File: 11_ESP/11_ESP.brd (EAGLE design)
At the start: 67.4 x 44.8 mm, 8 parts, among them T1 BC847, T2 BC847, X1 ALLSERIALSLAVE

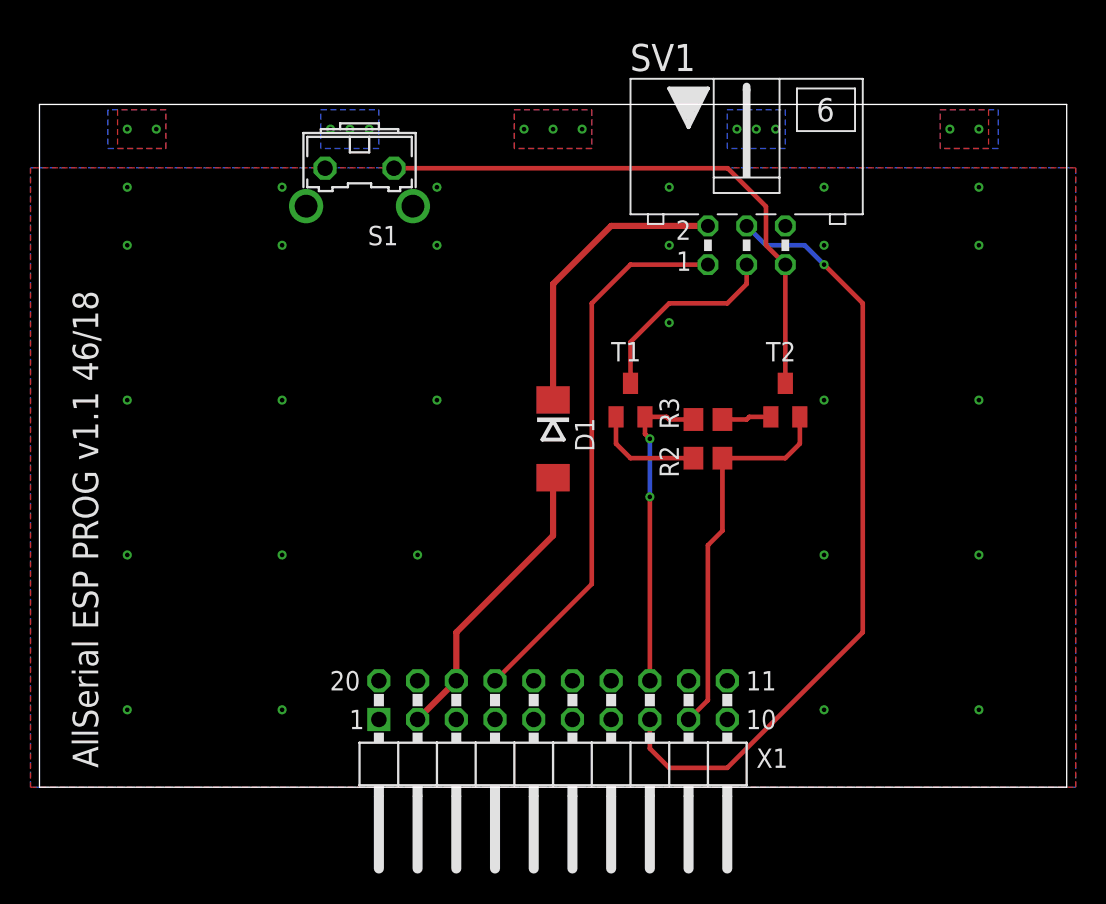
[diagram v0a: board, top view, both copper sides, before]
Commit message: Use lib elements
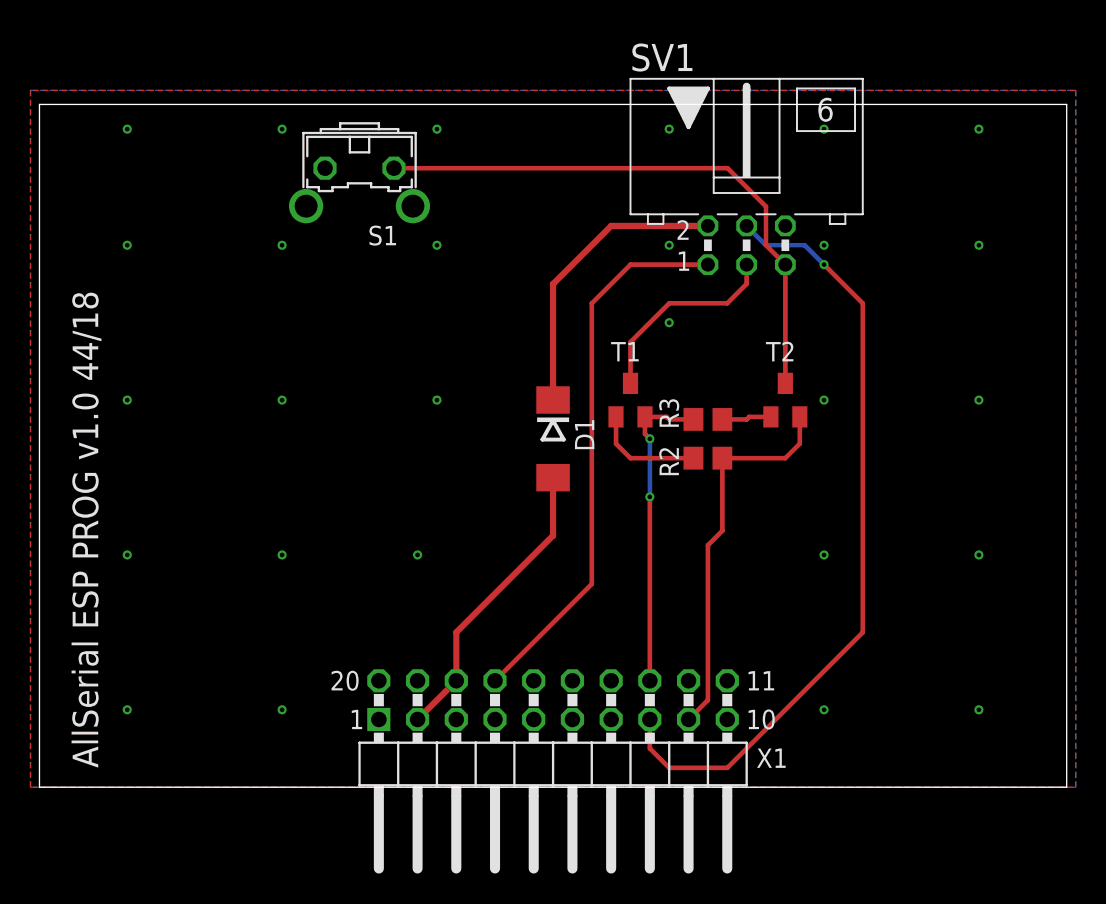
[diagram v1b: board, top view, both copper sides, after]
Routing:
- removed copper zone on layer 16, net N$10
- removed copper zone on layer 16, net N$11
- removed copper zone on layer 1, net N$13
- removed copper zone on layer 16, net N$13
- removed copper zone on layer 1, net N$14
- removed copper zone on layer 16, net N$14
- removed copper zone on layer 1, net N$15
- removed copper zone on layer 16, net N$15
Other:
- board text added: "AllSerial ESP PROG v1.0 44/18"
- board text removed: "AllSerial ESP PROG v1.1 46/18"
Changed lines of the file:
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@@
 <?xml version="1.0" encoding="utf-8"?>
 <!DOCTYPE eagle SYSTEM "eagle.dtd">
-<eagle version="7.7.0">
+<eagle version="7.6.0">
 <drawing>
 <settings>
@@
 <grid distance="1.27" unitdist="mm" unit="mm" style="lines" multiple="1" display="yes" altdistance="0.025" altunitdist="inch" altunit="inch"/>
 <layers>
-<layer number="1" name="Top" color="4" fill="1" visible="yes" active="yes"/>
+<layer number="1" name="Top" color="4" fill="1" visible="no" active="yes"/>
 <layer number="2" name="Route2" color="1" fill="3" visible="no" active="no"/>
 <layer number="3" name="Route3" color="4" fill="3" visible="no" active="no"/>
@@
 <layer number="14" name="Route14" color="1" fill="6" visible="no" active="no"/>
 <layer number="15" name="Route15" color="4" fill="6" visible="no" active="no"/>
-<layer number="16" name="Bottom" color="1" fill="1" visible="yes" active="yes"/>
+<layer number="16" name="Bottom" color="1" fill="1" visible="no" active="yes"/>
 <layer number="17" name="Pads" color="2" fill="1" visible="yes" active="yes"/>
-<layer number="18" name="Vias" color="2" fill="1" visible="yes" active="yes"/>
+<layer number="18" name="Vias" color="2" fill="1" visible="no" active="yes"/>
 <layer number="19" name="Unrouted" color="6" fill="1" visible="yes" active="yes"/>
 <layer number="20" name="Dimension" color="15" fill="1" visible="yes" active="yes"/>
@@
 <layer number="24" name="bOrigins" color="15" fill="1" visible="no" active="yes"/>
 <layer number="25" name="tNames" color="7" fill="1" visible="yes" active="yes"/>
-<layer number="26" name="bNames" color="7" fill="1" visible="yes" active="yes"/>
+<layer number="26" name="bNames" color="7" fill="1" visible="no" active="yes"/>
 <layer number="27" name="tValues" color="7" fill="1" visible="yes" active="yes"/>
 <layer number="28" name="bValues" color="7" fill="1" visible="no" active="yes"/>
-<layer number="29" name="tStop" color="7" fill="3" visible="yes" active="yes"/>
-<layer number="30" name="bStop" color="7" fill="6" visible="yes" active="yes"/>
+<layer number="29" name="tStop" color="7" fill="3" visible="no" active="yes"/>
+<layer number="30" name="bStop" color="7" fill="6" visible="no" active="yes"/>
 <layer number="31" name="tCream" color="7" fill="4" visible="no" active="yes"/>
 <layer number="32" name="bCream" color="7" fill="5" visible="no" active="yes"/>
@@
 <board>
 <plain>
-<text x="-29.845" y="1.27" size="1.6764" layer="21" rot="R90">AllSerial ESP PROG v1.1 46/18</text>
-<polygon width="0.254" layer="29">
-<vertex x="-25.4" y="44.45"/>
-<vertex x="-28.575" y="44.45"/>
-<vertex x="-28.575" y="41.91"/>
-<vertex x="-25.4" y="41.91"/>
-</polygon>
-<polygon width="0.254" layer="29">
-<vertex x="-2.54" y="44.45"/>
-<vertex x="2.54" y="44.45"/>
-<vertex x="2.54" y="41.91"/>
-<vertex x="-2.54" y="41.91"/>
-</polygon>
-<polygon width="0.254" layer="29">
-<vertex x="25.4" y="44.45"/>
-<vertex x="28.575" y="44.45"/>
-<vertex x="28.575" y="41.91"/>
-<vertex x="25.4" y="41.91"/>
-</polygon>
-<polygon width="0.254" layer="30">
-<vertex x="-29.21" y="44.45"/>
-<vertex x="-25.4" y="44.45"/>
-<vertex x="-25.4" y="41.91"/>
-<vertex x="-29.21" y="41.91"/>
-</polygon>
-<polygon width="0.254" layer="30">
-<vertex x="-15.24" y="44.45"/>
-<vertex x="-11.43" y="44.45"/>
-<vertex x="-11.43" y="41.91"/>
-<vertex x="-15.24" y="41.91"/>
-</polygon>
-<polygon width="0.254" layer="30">
-<vertex x="-2.54" y="44.45"/>
-<vertex x="2.54" y="44.45"/>
-<vertex x="2.54" y="41.91"/>
-<vertex x="-2.54" y="41.91"/>
-</polygon>
-<polygon width="0.254" layer="30">
-<vertex x="11.43" y="44.45"/>
-<vertex x="15.24" y="44.45"/>
-<vertex x="15.24" y="41.91"/>
-<vertex x="11.43" y="41.91"/>
-</polygon>
-<polygon width="0.254" layer="30">
-<vertex x="25.4" y="44.45"/>
-<vertex x="29.21" y="44.45"/>
-<vertex x="29.21" y="41.91"/>
-<vertex x="25.4" y="41.91"/>
-</polygon>
+<text x="-29.845" y="1.27" size="1.6764" layer="21" rot="R90">AllSerial ESP PROG v1.0 44/18</text>
+<rectangle x1="-8.89" y1="43.815" x2="-3.81" y2="45.72" layer="29"/>
+<rectangle x1="-25.4" y1="43.815" x2="-20.32" y2="45.72" layer="29"/>
+<rectangle x1="-1.27" y1="43.815" x2="3.81" y2="45.72" layer="29"/>
+<rectangle x1="21.59" y1="43.815" x2="26.67" y2="45.72" layer="29"/>
+<rectangle x1="-2.54" y1="43.815" x2="2.54" y2="45.72" layer="30"/>
+<rectangle x1="-12.7" y1="43.815" x2="-7.62" y2="45.72" layer="30"/>
+<rectangle x1="-22.86" y1="43.815" x2="-17.78" y2="45.72" layer="30"/>
+<rectangle x1="7.62" y1="43.815" x2="12.7" y2="45.72" layer="30"/>
+<rectangle x1="17.78" y1="43.815" x2="22.86" y2="45.72" layer="30"/>
 </plain>
 <attributes>
@@
 <signal name="GND">
 <polygon width="0.254" layer="16">
-<vertex x="-34.29" y="40.64"/>
-<vertex x="34.29" y="40.64"/>
+<vertex x="-34.29" y="45.72"/>
+<vertex x="34.29" y="45.72"/>
 <vertex x="34.29" y="0"/>
 <vertex x="-34.29" y="0"/>
@@
 <vertex x="-34.29" y="0"/>
 <vertex x="34.29" y="0"/>
-<vertex x="34.29" y="40.64"/>
-<vertex x="-34.29" y="40.64"/>
+<vertex x="34.29" y="45.72"/>
+<vertex x="-34.29" y="45.72"/>
 </polygon>
 <contactref element="X1" pad="1"/>
-<via x="-7.62" y="39.37" extent="1-16" drill="0.3"/>
-<via x="-17.78" y="39.37" extent="1-16" drill="0.3"/>
-<via x="-27.94" y="39.37" extent="1-16" drill="0.3"/>
+<via x="-7.62" y="43.18" extent="1-16" drill="0.3"/>
+<via x="-17.78" y="43.18" extent="1-16" drill="0.3"/>
+<via x="-27.94" y="43.18" extent="1-16" drill="0.3"/>
 <via x="-27.94" y="35.56" extent="1-16" drill="0.3"/>
 <via x="-17.78" y="35.56" extent="1-16" drill="0.3"/>
@@
 <via x="7.62" y="30.48" extent="1-16" drill="0.3"/>
 <via x="7.62" y="35.56" extent="1-16" drill="0.3"/>
-<via x="7.62" y="39.37" extent="1-16" drill="0.3"/>
-<via x="17.78" y="39.37" extent="1-16" drill="0.3"/>
+<via x="7.62" y="43.18" extent="1-16" drill="0.3"/>
+<via x="17.78" y="43.18" extent="1-16" drill="0.3"/>
 <via x="17.78" y="35.56" extent="1-16" drill="0.3"/>
-<via x="27.94" y="39.37" extent="1-16" drill="0.3"/>
+<via x="27.94" y="43.18" extent="1-16" drill="0.3"/>
 <via x="27.94" y="35.56" extent="1-16" drill="0.3"/>
 <via x="17.78" y="25.4" extent="1-16" drill="0.3"/>
@@
 <wire x1="6.35" y1="2.54" x2="6.35" y2="4.445" width="0.3048" layer="1"/>
 </signal>
-<signal name="N$13">
-<polygon width="0.254" layer="16">
-<vertex x="-25.4" y="44.45"/>
-<vertex x="-29.21" y="44.45"/>
-<vertex x="-29.21" y="41.91"/>
-<vertex x="-25.4" y="41.91"/>
-</polygon>
-<polygon width="0.254" layer="1">
-<vertex x="-25.4" y="44.45"/>
-<vertex x="-28.575" y="44.45"/>
-<vertex x="-28.575" y="41.91"/>
-<vertex x="-25.4" y="41.91"/>
-</polygon>
-<via x="-26.035" y="43.18" extent="1-16" drill="0.3"/>
-<via x="-27.94" y="43.18" extent="1-16" drill="0.3"/>
-</signal>
-<signal name="N$14">
-<polygon width="0.254" layer="16">
-<vertex x="-2.54" y="44.45"/>
-<vertex x="2.54" y="44.45"/>
-<vertex x="2.54" y="41.91"/>
-<vertex x="-2.54" y="41.91"/>
-</polygon>
-<polygon width="0.254" layer="1">
-<vertex x="-2.54" y="44.45"/>
-<vertex x="2.54" y="44.45"/>
-<vertex x="2.54" y="41.91"/>
-<vertex x="-2.54" y="41.91"/>
-</polygon>
-<via x="0" y="43.18" extent="1-16" drill="0.3"/>
-<via x="-1.905" y="43.18" extent="1-16" drill="0.3"/>
-<via x="1.905" y="43.18" extent="1-16" drill="0.3"/>
-</signal>
-<signal name="N$15">
-<polygon width="0.254" layer="16">
-<vertex x="25.4" y="44.45"/>
-<vertex x="29.21" y="44.45"/>
-<vertex x="29.21" y="41.91"/>
-<vertex x="25.4" y="41.91"/>
-</polygon>
-<polygon width="0.254" layer="1">
-<vertex x="25.4" y="44.45"/>
-<vertex x="28.575" y="44.45"/>
-<vertex x="28.575" y="41.91"/>
-<vertex x="25.4" y="41.91"/>
-</polygon>
-<via x="26.035" y="43.18" extent="1-16" drill="0.3"/>
-<via x="27.94" y="43.18" extent="1-16" drill="0.3"/>
-</signal>
-<signal name="N$10">
-<polygon width="0.254" layer="16">
-<vertex x="-15.24" y="44.45"/>
-<vertex x="-11.43" y="44.45"/>
-<vertex x="-11.43" y="41.91"/>
-<vertex x="-15.24" y="41.91"/>
-</polygon>
-<via x="-13.335" y="43.18" extent="1-16" drill="0.3"/>
-<via x="-14.605" y="43.18" extent="1-16" drill="0.3"/>
-<via x="-12.065" y="43.18" extent="1-16" drill="0.3"/>
-</signal>
-<signal name="N$11">
-<polygon width="0.254" layer="16">
-<vertex x="11.43" y="44.45"/>
-<vertex x="15.24" y="44.45"/>
-<vertex x="15.24" y="41.91"/>
-<vertex x="11.43" y="41.91"/>
-</polygon>
-<via x="13.335" y="43.18" extent="1-16" drill="0.3"/>
-<via x="12.065" y="43.18" extent="1-16" drill="0.3"/>
-<via x="14.605" y="43.18" extent="1-16" drill="0.3"/>
-</signal>
 </signals>
